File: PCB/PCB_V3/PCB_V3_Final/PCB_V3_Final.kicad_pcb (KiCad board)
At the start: 2 copper layers, 84 parts, among them J1 ESP_Left, J10 LHS_Arrow_+ve, J11 MCP_B0, J12 LHS_Arrow_-ve, J13 ACS2_Screw, J14 ACS4_Screw, J15 LAN8720_pins_2, J16 LAN8720_pins_1, J17 MCP_VCC_LINE, J18 RHS_Arrow_+ve, J19 RHS_Arrow_-ve, J2 ESP_Right, J20 AMS_IP_Pins, J21 BC1_IN+, J22 BC1_IN-, J23 BC3_IN+, J24 BC3_IN-, J25 AMS_OP_Pins, J26 BC1_OUT+, J27 BC1_OUT-, J28 BC3_OUT+, J29 BC3_OUT-, J3 ACS1_Pins, J30 STATIC_LED_1, J31 STATIC_LED_2, J32 BC2_IN+, J33 BC2_IN-, J34 BC5_IN+, J35 BC5_IN-, J36 I/P_Terminal, J37 Battery_Terminal, J38 BC2_OUT+, J39 BC2_OUT-, J4 ACS3_Pins, J40 BC5_OUT+, J41 BC5_OUT-, J5 ACS3_Screw, J6 ACS1_Screw, J7 ACS2_pins, J8 MCP_A0, J9 ACS4_Pins, Q1 IRLZ44N, Q10 IRLZ44N, Q2 IRLZ44N, Q3 IRLZ44N, Q4 IRLZ44N, Q5 IRLZ44N, Q6 IRLZ44N, Q7 IRLZ44N, Q8 IRLZ44N, Q9 IRLZ44N

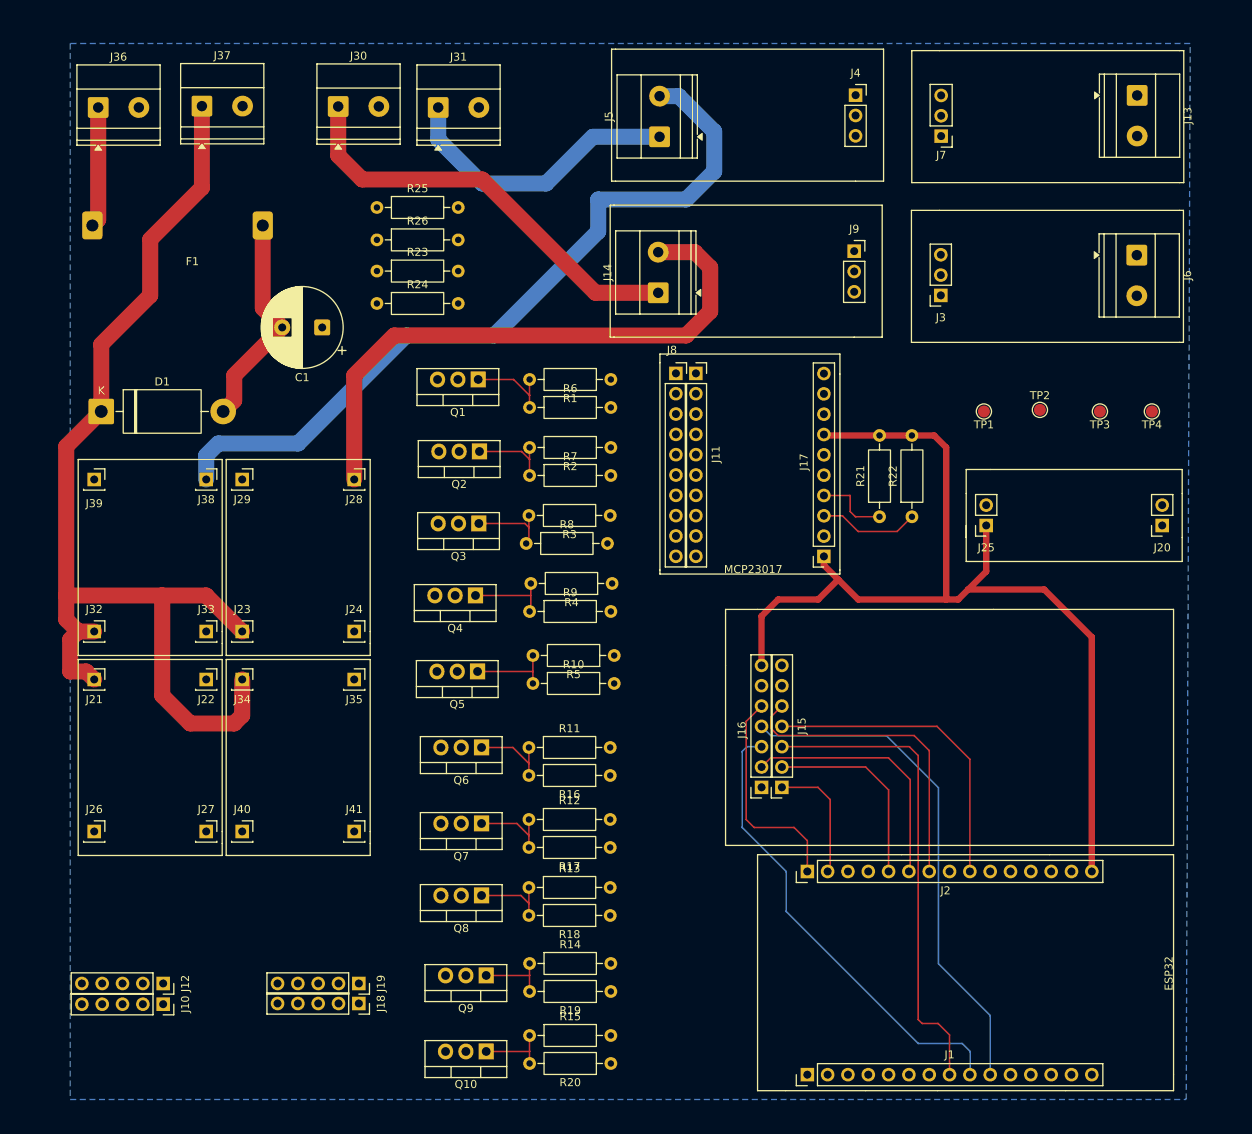
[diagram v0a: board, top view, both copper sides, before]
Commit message: Uploading the final PCB files
1. Finished product
2. Made the remaining connections
3. Added the mounting holes for the PCB
4. Final producct --> has to be reviewed in the meeting
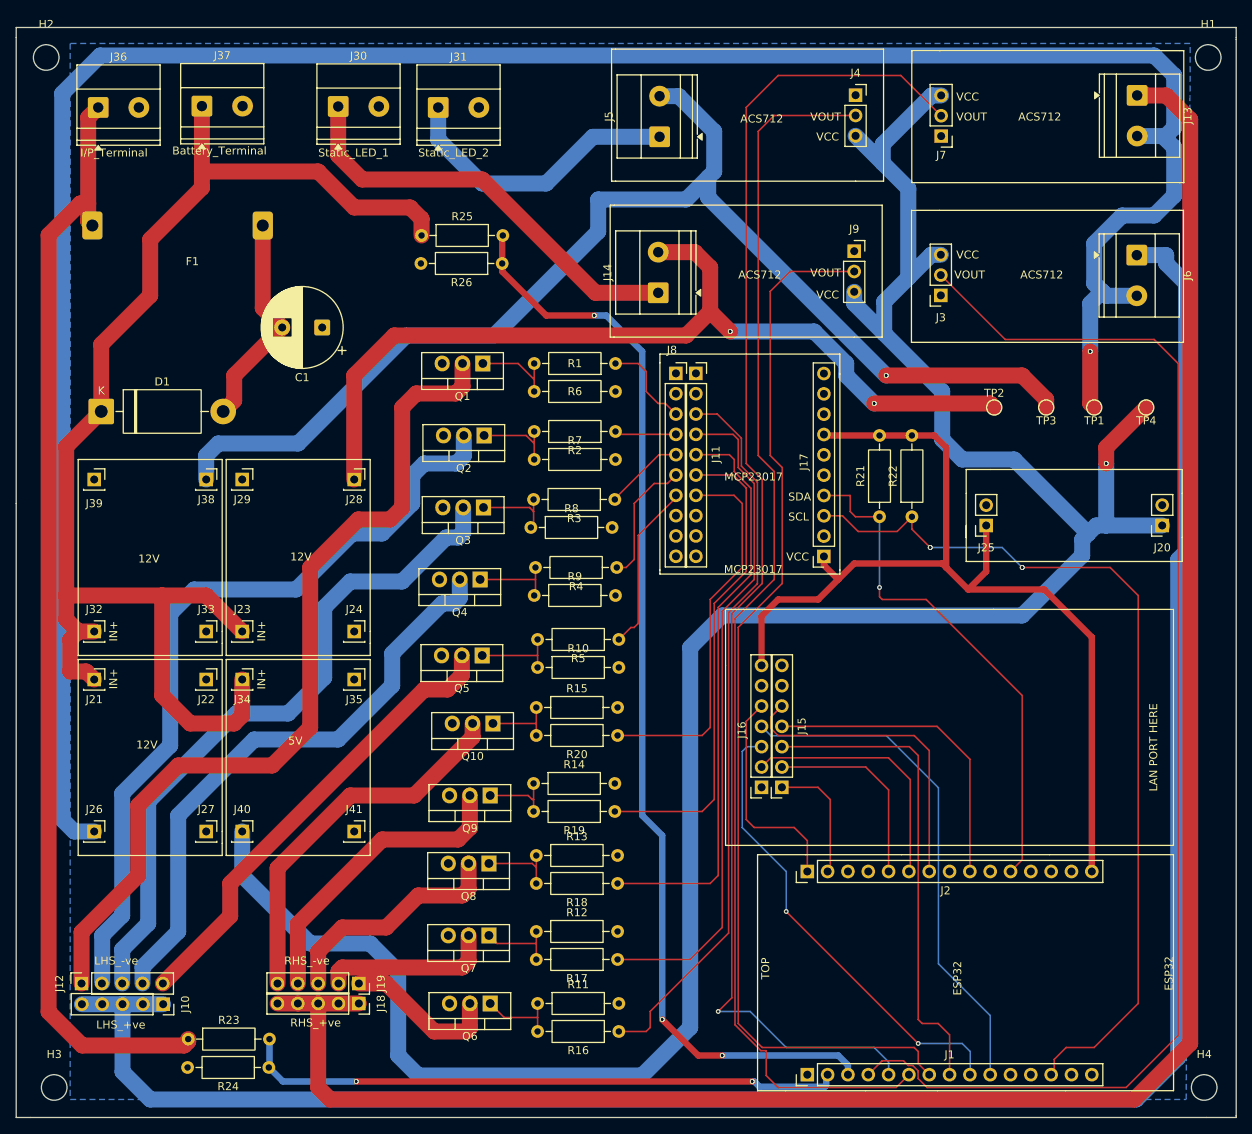
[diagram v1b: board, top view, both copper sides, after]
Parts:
- added H1: MountingScrew, MountingHole:MountingHole_3.2mm_M3, F.Cu at (219.8, 25.2)
- added H2: MountingScrew, MountingHole:MountingHole_3.2mm_M3, F.Cu at (74.5, 25.2)
- added H3: MountingScrew, MountingHole:MountingHole_3.2mm_M3, F.Cu at (75.5, 154.0)
- added H4: MountingScrew, MountingHole:MountingHole_3.2mm_M3, F.Cu at (219.2, 154.0)
- moved R23 98.9 mm to (92.2, 147.9)
- moved R24 96.5 mm to (102.3, 151.5), turned to 180 degrees
- moved Q10 41.0 mm to (130.3, 108.5)
- moved R15 41.0 mm to (135.8, 106.5)
- moved R20 41.0 mm to (145.9, 110.0)
- moved Q6 32.0 mm to (130.0, 143.5)
- moved R11 32.0 mm to (135.9, 143.5)
- moved R16 32.0 mm to (146.1, 147.0)
- moved Q9 22.5 mm to (130.0, 117.5)
- moved R14 22.5 mm to (135.4, 116.0)
- moved R19 22.5 mm to (145.6, 119.5)
- moved R26 15.9 mm to (131.5, 51.0), turned to 180 degrees
- moved Q7 14.0 mm to (129.8, 135.0)
- moved R12 14.0 mm to (135.8, 134.5)
- moved R17 14.0 mm to (145.9, 138.0)
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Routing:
- net /5V: track 0.00 -> 303.5 mm, vias 0 -> 2
- net /12V_LR: track 0.00 -> 295.6 mm, vias 0 -> 2
- net /LHS_LED_IP+: track 0.00 -> 259.6 mm
- net /RHS_LED_IP+: track 0.00 -> 256.6 mm
- net /D35: track 0.00 -> 169.7 mm, vias 0 -> 1
- net /D34: track 0.00 -> 162.4 mm
- net /D32: track 0.00 -> 155.0 mm
- net /BATT_VD: track 0.00 -> 137.5 mm, vias 0 -> 6
- net /D33: track 0.00 -> 133.4 mm
- net /14.5: track 15.1 -> 138.9 mm
- net /LHS_LED_1: track 0.00 -> 109.3 mm
- net /D13: track 12.6 -> 112.3 mm, vias 0 -> 4
- net /LHS_LED_2: track 0.00 -> 99.1 mm
- net /B0: track 0.00 -> 91.1 mm
- net /LHS_LED_3: track 0.00 -> 85.6 mm
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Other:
- board outline added: 152.5 x 136.2 mm
- board text added: "12V"
- board text added: "5V"
- board text added: "ACS712"
- board text added: "Battery_Terminal"
- board text added: "I/P_Terminal"
- board text added: "IN+"
- board text added: "LAN PORT HERE"
- board text added: "LHS_+ve"
- board text added: "LHS_-ve"
- board text added: "RHS_+ve"
- board text added: "RHS_-ve"
- board text added: "SCL"
- board text added: "SDA"
- board text added: "Static_LED_1"
- board text added: "Static_LED_2"
- board text added: "TOP"
- board text added: "VCC"
- board text added: "VOUT"
